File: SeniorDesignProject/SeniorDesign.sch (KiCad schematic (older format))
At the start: 22 parts, among them J1 RJ45(LoadCells), J2 RJ45(Accelerometer), J3 PICkit3, J4 RJ11(ICD3), J5 ID-12LA Header, J6 XBEE Header, P7 Power 1, P9 Power 2, U1 INA827, U10 7905, U9 7805

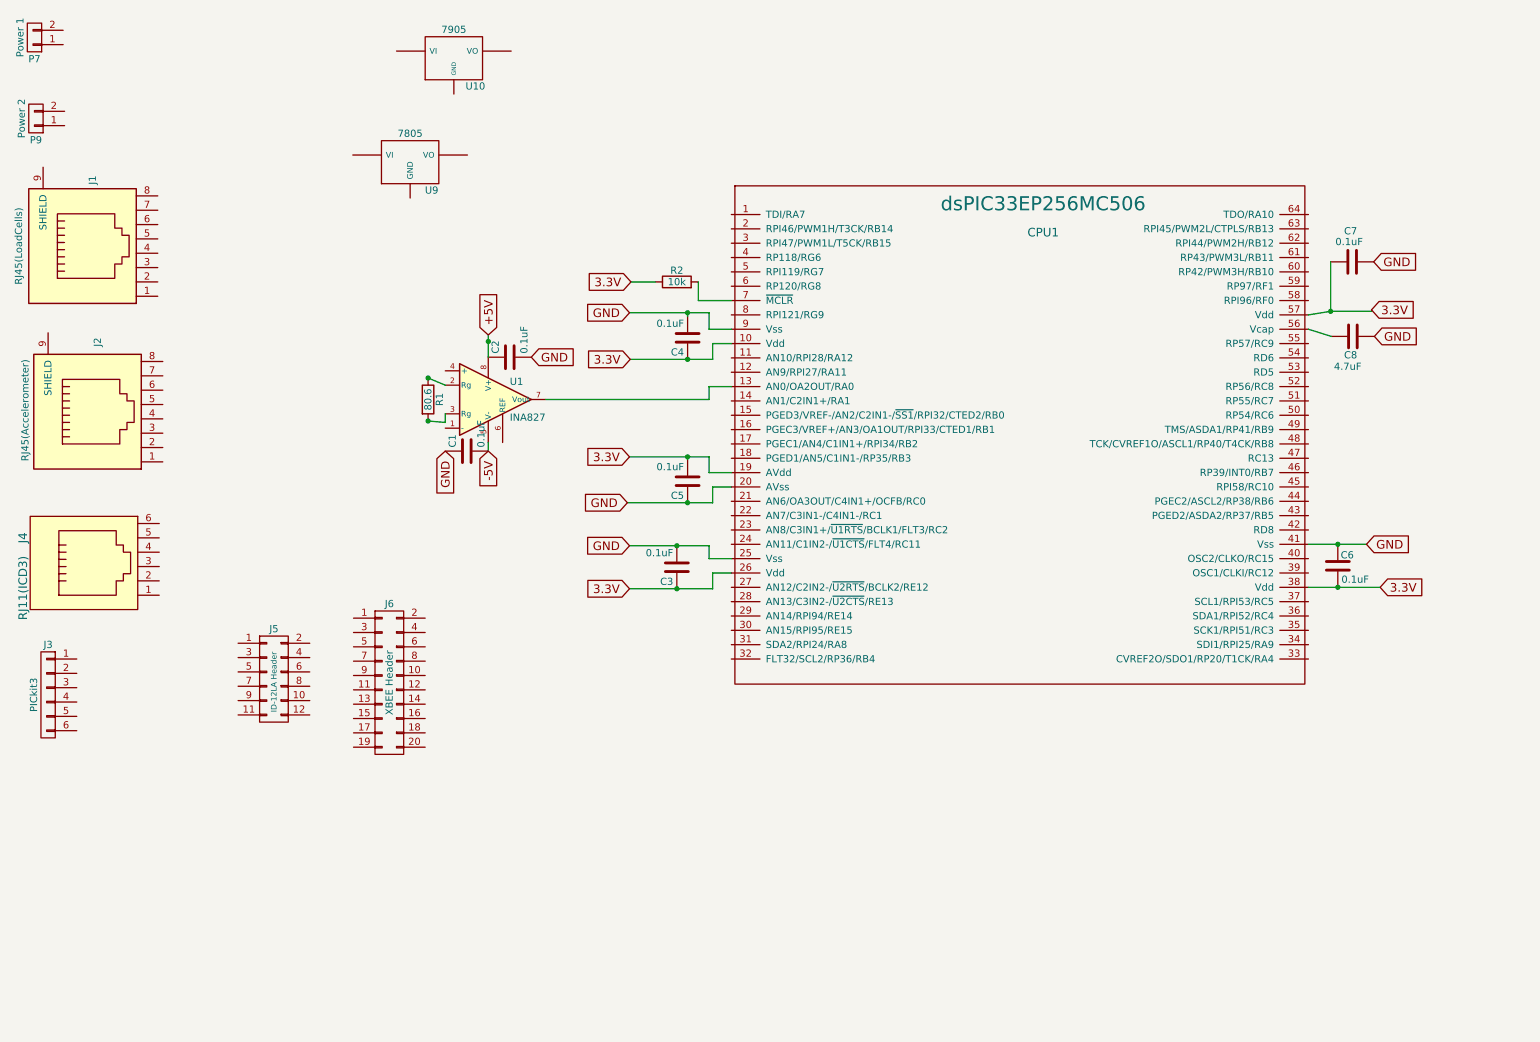
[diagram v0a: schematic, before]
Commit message: Updates
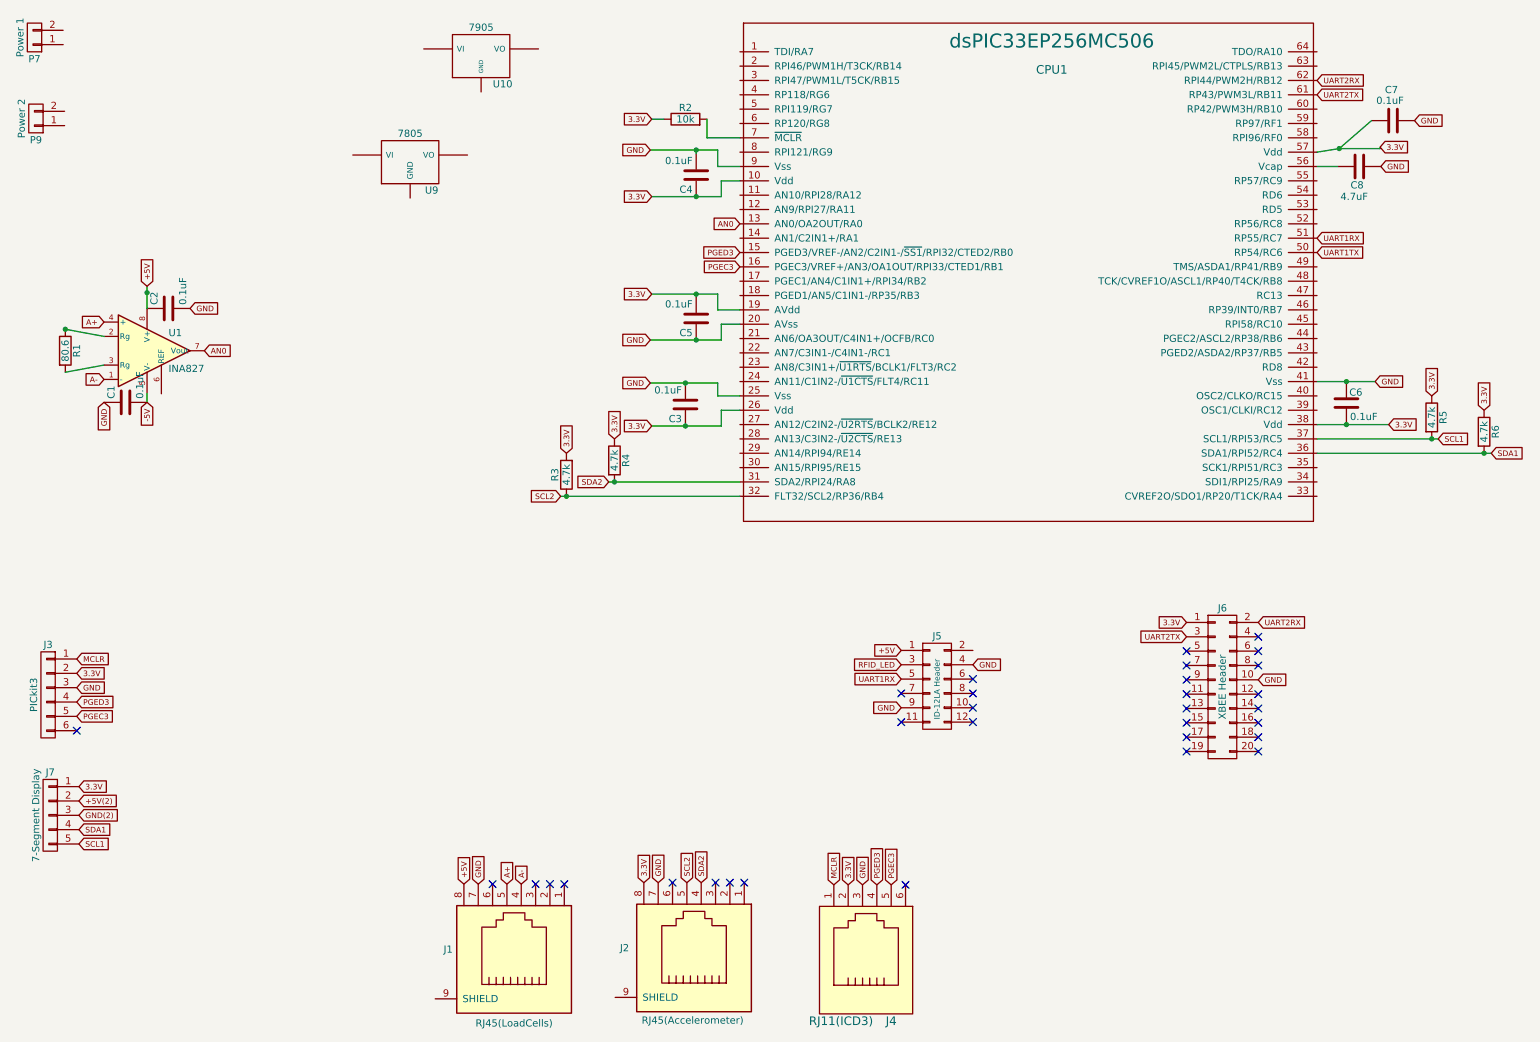
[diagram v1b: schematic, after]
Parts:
- added J7: 7-Segment Display, Socket_Strips:Socket_Strip_Straight_1x05_Pitch2.54mm, symbol CONN_01X05
- added R3, R4, R5, R6: 4.7k, Resistors_SMD:R_0805, symbol R
- U10, U9: footprint TO_SOT_Packages_THT:TO-220_Neutral123_Vertical -> TO_SOT_Packages_THT:TO-220_Horizontal
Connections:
- net +5V: now also J1.8, J5.1 (P1)
- net 3.3V: now also J2.8, J3.2 (P2), J4.2, J6.1 (P1), J7.1 (P1), R3.2, R4.1, R5.1, R6.1
- net GND: now also J1.7, J2.7, J3.3 (P3), J4.3, J5.4 (P4), J5.9 (P9), J6.10 (P10)
- net AN0: now reaches CPU1.13 (AN0/OA2OUT/RA0), U1.7 (Vout)
- net PGED3: now reaches CPU1.15 (PGED3/VREF-/AN2/C2IN1-/~SS1~/RPI32/CTED2/RB0)
- net PGED3: now also J3.4 (P4), J4.4
- net PGEC3: now reaches CPU1.16 (PGEC3/VREF+/AN3/OA1OUT/RPI33/CTED1/RB1)
- net PGEC3: now also J3.5 (P5), J4.5
- net SDA2: now reaches CPU1.31 (SDA2/RPI24/RA8)
- net SDA2: now also J2.4, R4.2
- net SCL2: now reaches CPU1.32 (FLT32/SCL2/RP36/RB4)
- net SCL2: now also J2.5, R3.1
- net SDA1: now reaches CPU1.36 (SDA1/RPI52/RC4)
- net SDA1: now also J7.4 (P4), R6.2
- net SCL1: now reaches CPU1.37 (SCL1/RPI53/RC5)
- net SCL1: now also J7.5 (P5), R5.2
- net UART1TX: now reaches CPU1.50 (RP54/RC6)
- net UART1RX: now reaches CPU1.51 (RP55/RC7)
- net UART1RX: now also J5.5 (P5)
- net UART2TX: now reaches CPU1.61 (RP43/PWM3L/RB11)
- net UART2TX: now also J6.3 (P3)
- net UART2RX: now reaches CPU1.62 (RPI44/PWM2H/RB12)
- net UART2RX: now also J6.2 (P2)
- net A-: now reaches J1.4
- net A-: now also U1.1 (-)
- net A+: now reaches J1.5
- net A+: now also U1.4 (+)
- net RFID_LED: now reaches J5.3 (P3)
- net MCLR: now reaches J4.1
- net MCLR: now also J3.1 (P1)
- new net +5V(2): J7.2 (P2)
- new net GND(2): J7.3 (P3)
- no-connect marks 0 -> 32
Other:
- moved on the sheet: C1, C2, C3, C4, C5, C6, C7, C8, CPU1, J1, J2, J4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
